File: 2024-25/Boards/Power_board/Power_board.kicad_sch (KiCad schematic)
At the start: 28 parts, among them J1 430451001, J2 430451001, Q1 AON6411, Q2 AON6411, Q3 AON6411, Q4 AON6411, Q5 AON6411

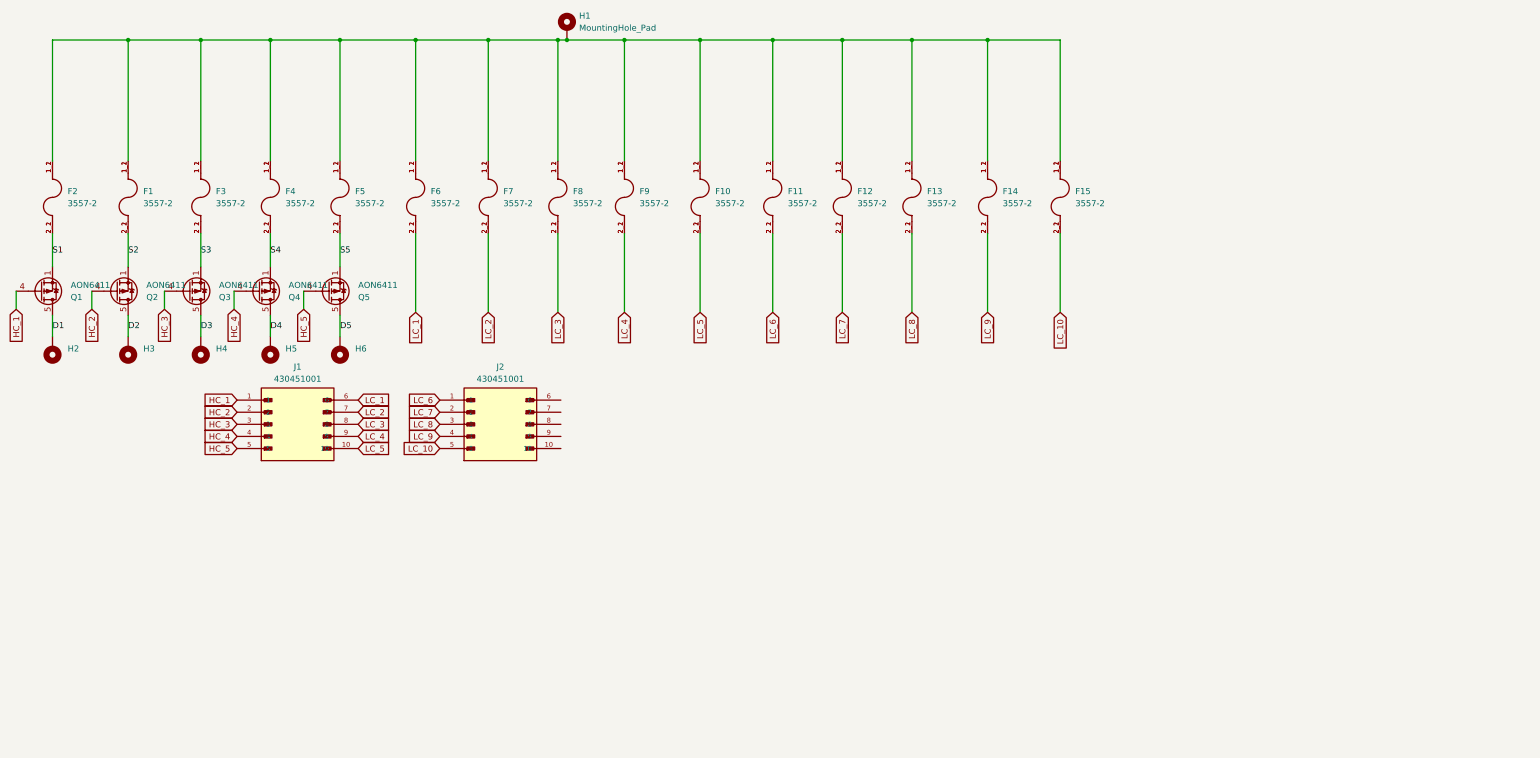
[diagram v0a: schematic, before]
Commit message: organizational changes
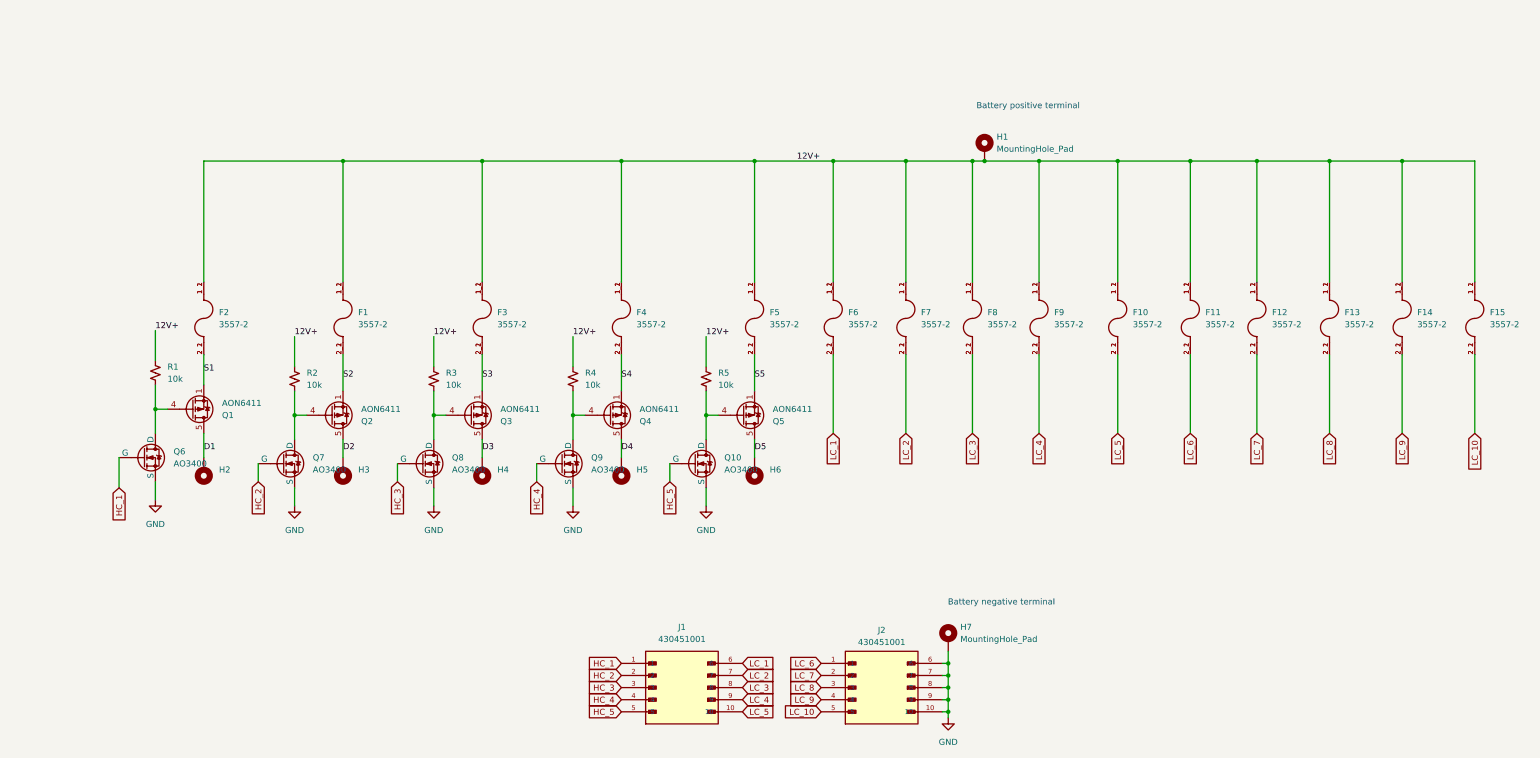
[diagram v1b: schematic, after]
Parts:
- added H7: MountingHole_Pad, MountingHole:MountingHole_5.3mm_M5_Pad, symbol Mechanical:MountingHole_Pad
- added Q10, Q6, Q7, Q8, Q9: AO3400, Package_TO_SOT_SMD:SOT-23-3, symbol Simulation_SPICE:NMOS
- added R1, R2, R3, R4, R5: 10k, symbol Device:R_Small_US
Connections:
- net HC_1: now also Q6.2 (G); no longer Q1.4 (G)
- net HC_2: now also Q7.2 (G); no longer Q2.4 (G)
- net HC_3: now also Q8.2 (G); no longer Q3.4 (G)
- net HC_4: now also Q9.2 (G); no longer Q4.4 (G)
- net HC_5: now also Q10.2 (G); no longer Q5.4 (G)
- net 12V+: now reaches F1.1_1, F1.1_2, F10.1_1, F10.1_2, F11.1_1, F11.1_2, F12.1_1, F12.1_2, F13.1_1, F13.1_2, F14.1_1, F14.1_2, F15.1_1, F15.1_2, F2.1_1, F2.1_2, F3.1_1, F3.1_2, F4.1_1, F4.1_2, F5.1_1, F5.1_2, F6.1_1, F6.1_2, F7.1_1, F7.1_2, F8.1_1, F8.1_2, F9.1_1, F9.1_2, H1.1
- net 12V+: now also R1.1, R2.1, R3.1, R4.1, R5.1
- net GND: now reaches J2.10
- net GND: now also J2.6, J2.7, J2.8, J2.9, H7.1, Q10.3 (S), Q6.3 (S), Q7.3 (S), Q8.3 (S), Q9.3 (S)
- new net: Q4.4 (G), Q9.1 (D), R4.2
- new net: Q1.4 (G), Q6.1 (D), R1.2
- new net: Q2.4 (G), Q7.1 (D), R2.2
- new net: Q10.1 (D), Q5.4 (G), R5.2
- new net: Q3.4 (G), Q8.1 (D), R3.2
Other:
- note added: "Battery negative terminal"
- note added: "Battery positive terminal"
- moved on the sheet: F1, F10, F11, F12, F13, F14, F15, F2, F3, F4, F5, F6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
